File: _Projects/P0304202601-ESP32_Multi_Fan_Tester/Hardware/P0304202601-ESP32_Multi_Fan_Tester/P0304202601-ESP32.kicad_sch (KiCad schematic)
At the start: 10 parts, among them CN2 KHS4B-PH-SM4-TB(LF)(SN), IC2 ESP32-WROOM-32UE-N16

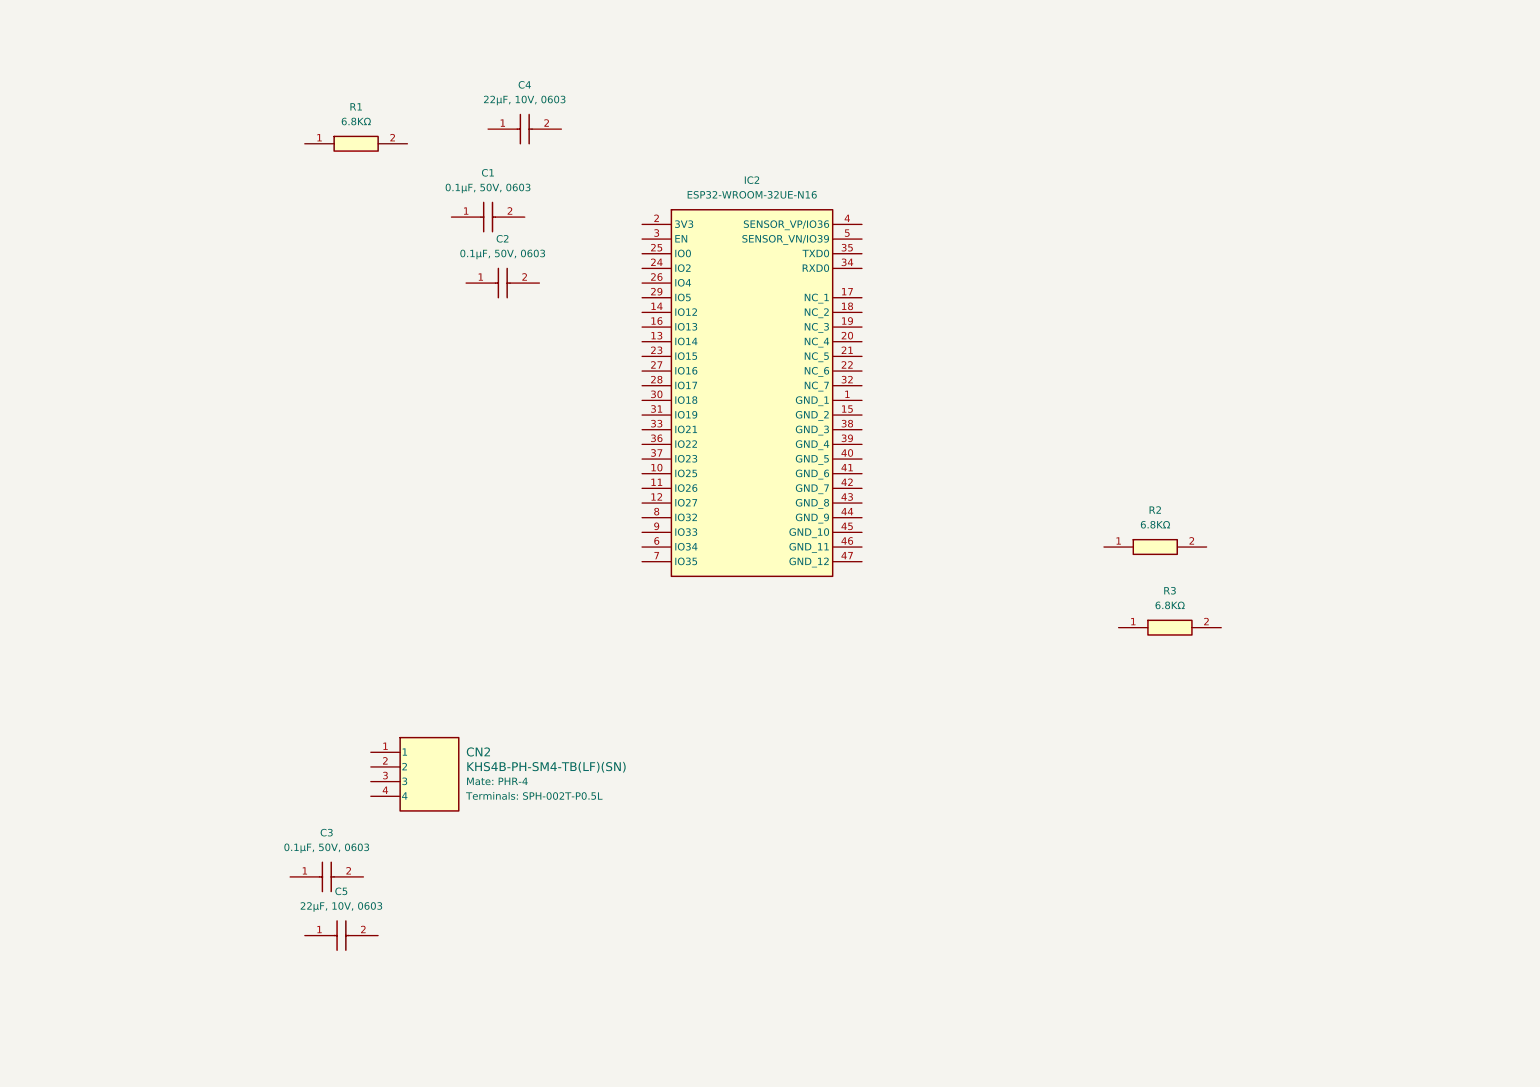
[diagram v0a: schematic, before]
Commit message: Added new content from recent stream.
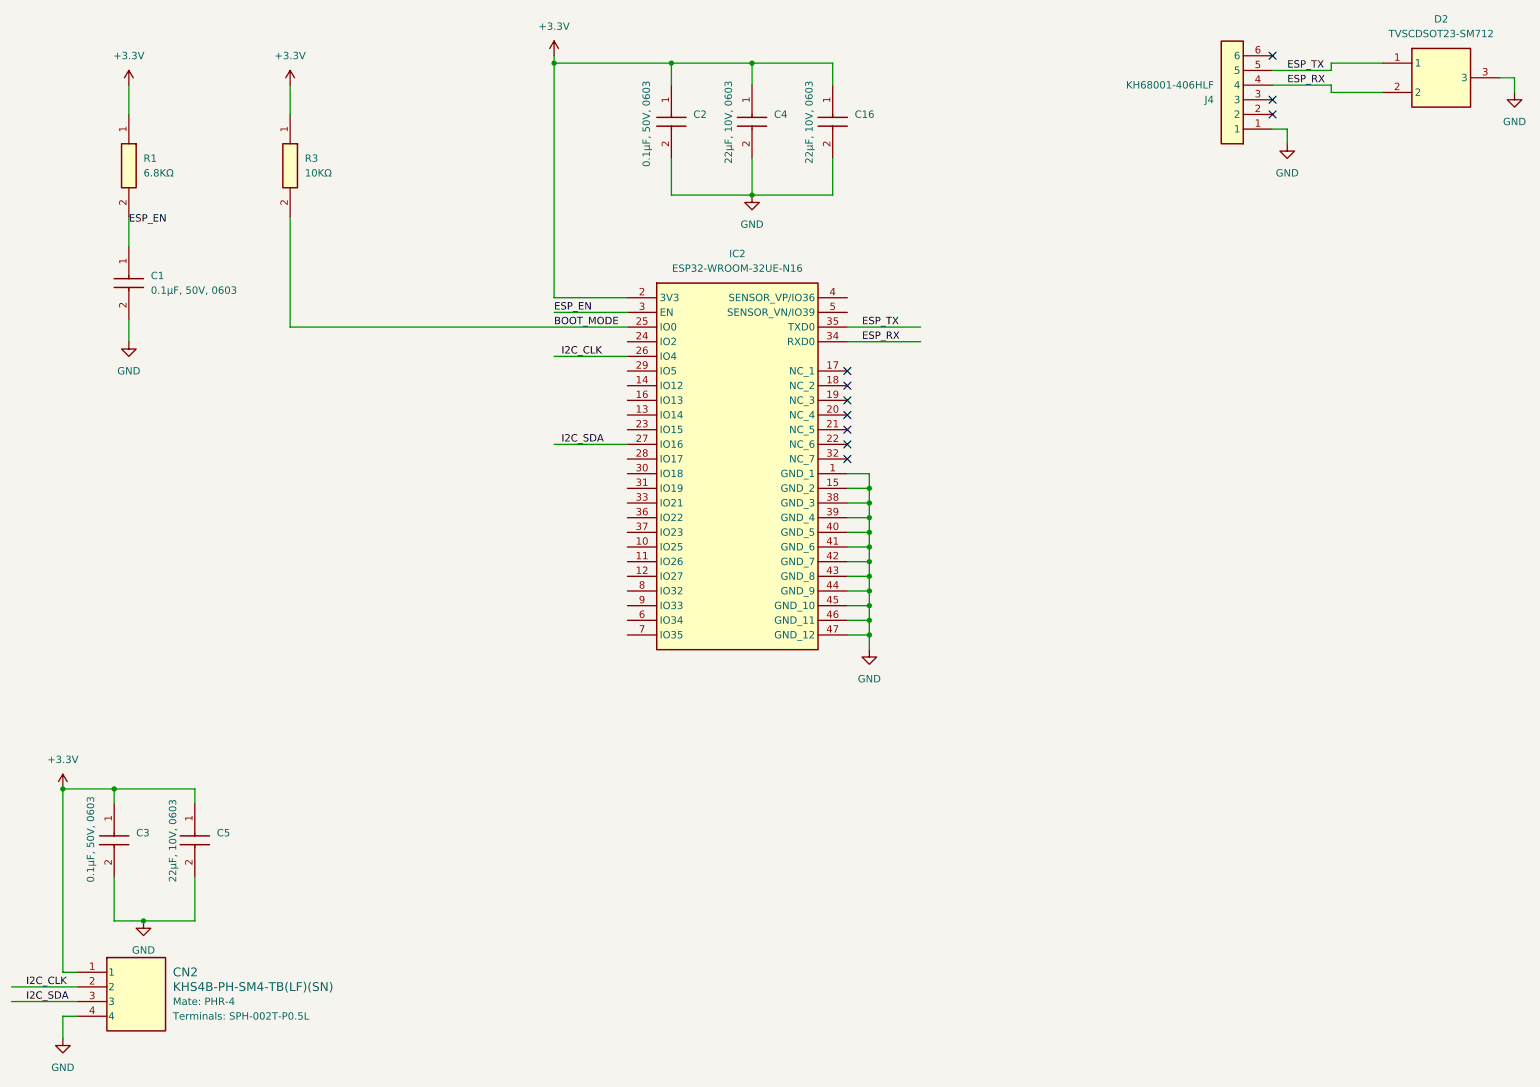
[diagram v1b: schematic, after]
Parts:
- removed R2, R3: RC0603682075AAA, COMPONENTS:RES-0603, symbol COMPONENTS:RC0603682075AAA
- added C16: CC0603226010AABX5R, COMPONENTS:CAP-0603, symbol COMPONENTS:CC0603226010AABX5R
- added D2: TVSCDSOT23-SM712, COMPONENTS:SOT-23-3, symbol COMPONENTS:TVSCDSOT23-SM712
- added J4: KH68001-406HLF, CONNECTORS:6x1HDR2.54mm, symbol CONNECTORS:KH68001-406HLF
- added R3: RC060310K2075AAA, COMPONENTS:RES-0603, symbol COMPONENTS:RC060310K2075AAA
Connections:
- net +3.3V: now reaches R1.1
- net +3.3V: now also C2.1, C3.1, C4.1, C5.1, CN2.1, IC2.2 (3V3), C16.1, R3.1
- net ESP_EN: now reaches R1.2
- net ESP_EN: now also C1.1, IC2.3 (EN)
- net GND: now reaches C5.2
- net GND: now also C1.2, C2.2, C3.2, C4.2, CN2.4, IC2.1 (GND_1), IC2.15 (GND_2), IC2.38 (GND_3), IC2.39 (GND_4), IC2.40 (GND_5), IC2.41 (GND_6), IC2.42 (GND_7), IC2.43 (GND_8), IC2.44 (GND_9), IC2.45 (GND_10), IC2.46 (GND_11), IC2.47 (GND_12), C16.2, D2.3, J4.1
- net I2C_CLK: now reaches CN2.2
- net I2C_CLK: now also IC2.26 (IO4)
- net I2C_SDA: now reaches CN2.3
- net I2C_SDA: now also IC2.27 (IO16)
- net BOOT_MODE: now reaches IC2.25 (IO0)
- net BOOT_MODE: now also R3.2
- net ESP_RX: now reaches IC2.34 (RXD0)
- net ESP_RX: now also D2.2, J4.4
- net ESP_TX: now reaches IC2.35 (TXD0)
- net ESP_TX: now also D2.1, J4.5
- no-connect marks 0 -> 10
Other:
- moved on the sheet: C1, C2, C3, C4, C5, CN2, IC2, R1
